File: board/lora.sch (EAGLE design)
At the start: 32 parts, among them IC1 STM32F030F4, IC2 ADP1607, J1 SWD_PTH_SHROUD, X1 SMA-142-0701-801/806, X2 UBLOX_MAX, X3 RFM98

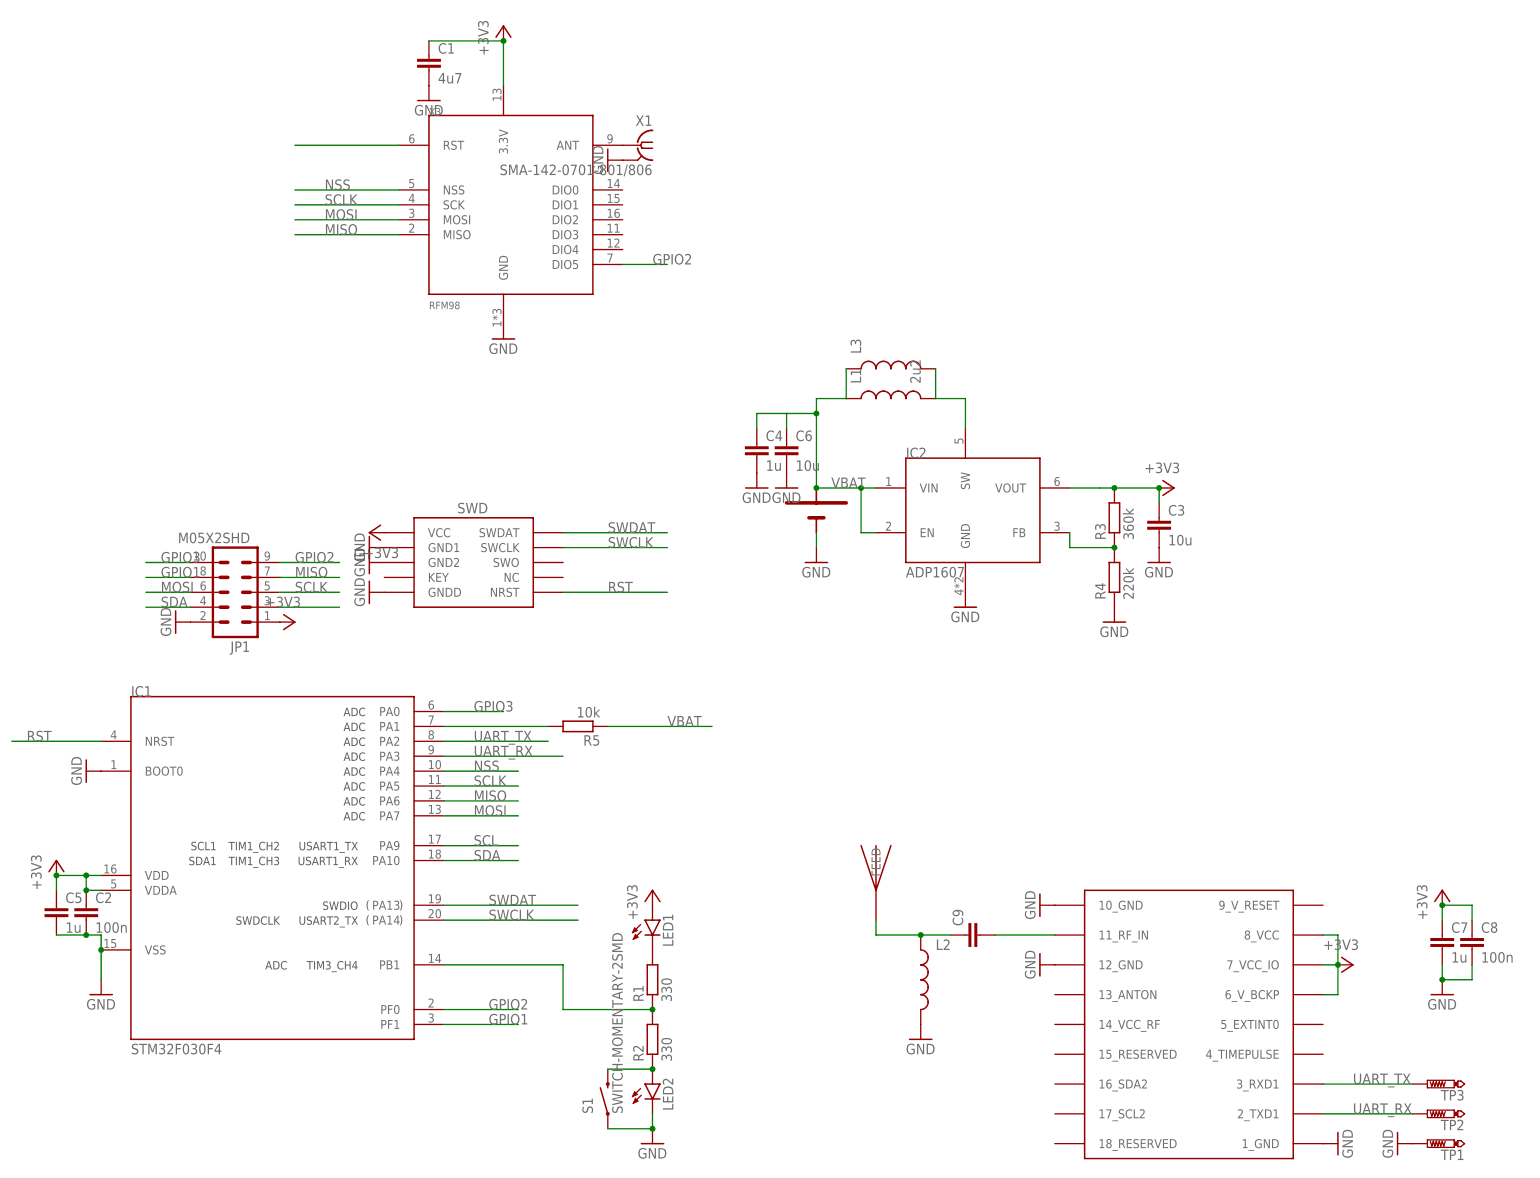
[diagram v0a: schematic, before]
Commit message: improvments
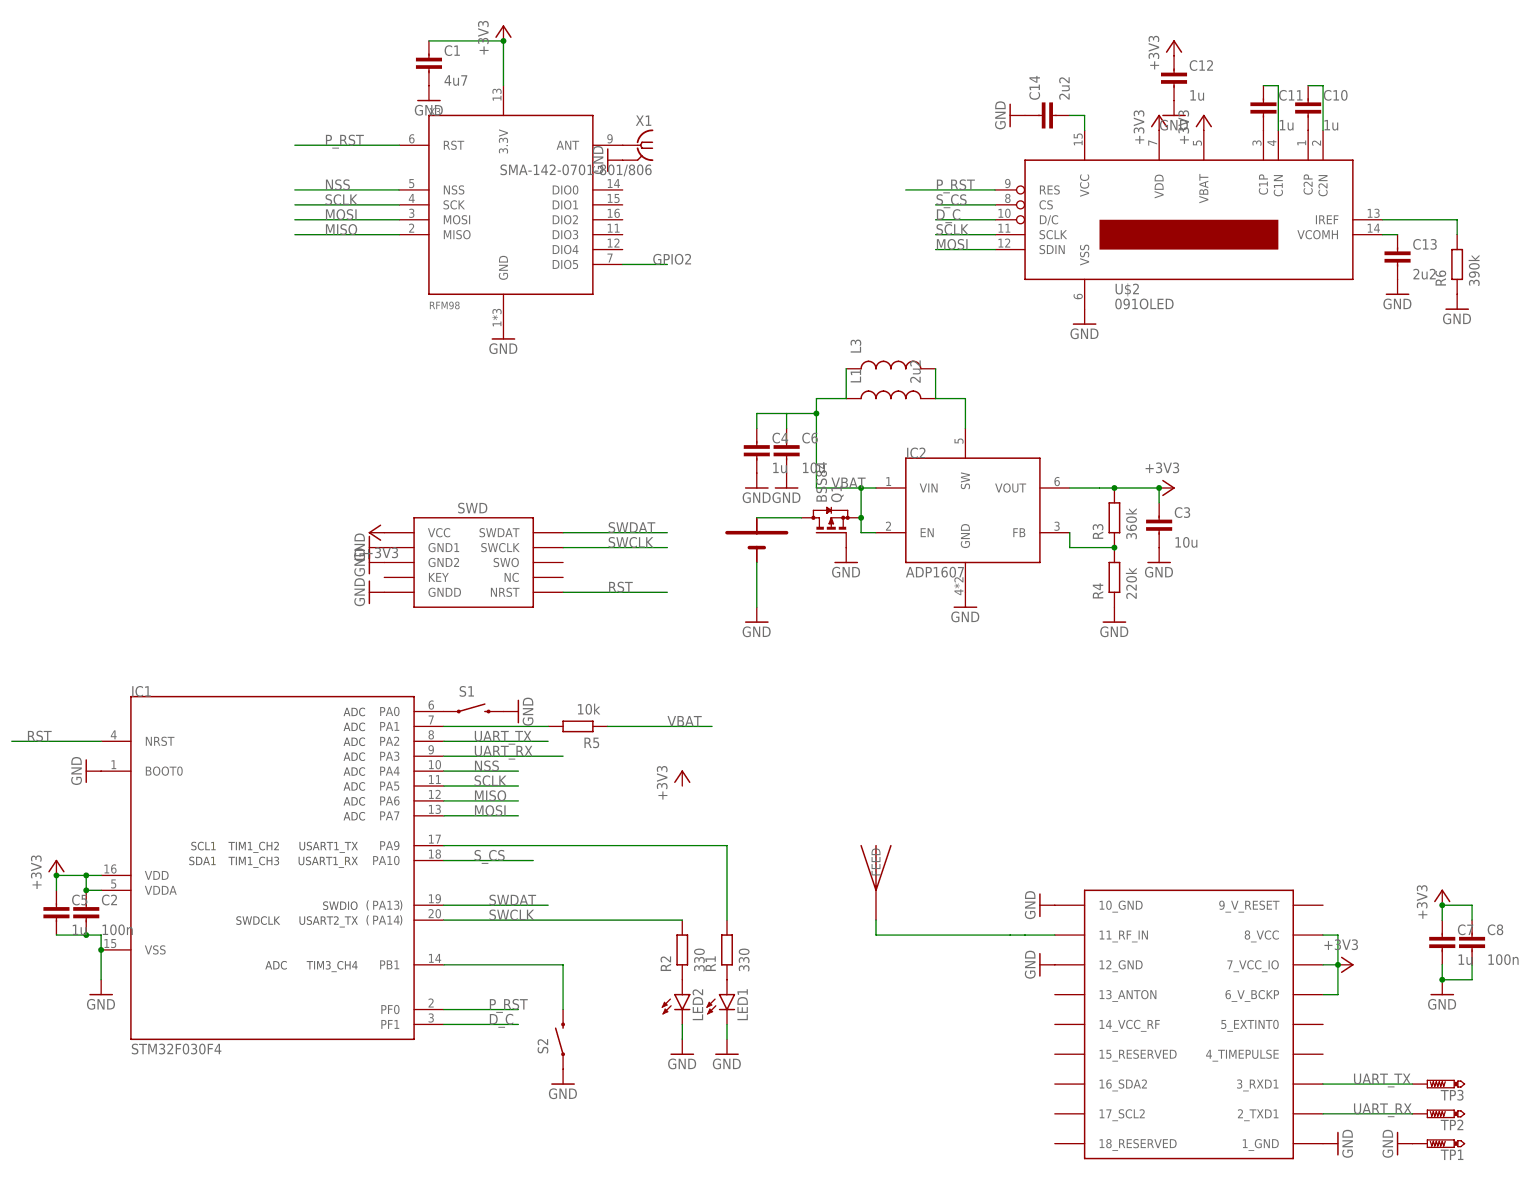
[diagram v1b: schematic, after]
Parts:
- removed C9: (no value), rcl:C-EUC0603
- removed JP1: M05X2SHD, SparkFun-Connectors:M05X2SHD
- removed L2: (no value), SparkFun-Passives:INDUCTOR0603
- added C10, C11, C12: 1u, passives-7351:CAPACITOR0603-N
- added C13, C14: 2u2, passives-7351:CAPACITOR0603-N
- added Q1: BSS84, transistor-small-signal:BSS84
- added R6: 390k, passives-7351:RESISTOR0603-N
- added S2: SWITCH-MOMENTARY-2SMD, Mine:SWITCH-MOMENTARY-2SMD
- added U$2: 091OLED, ukhas:091OLED
- C1, C2, C4, C5, C7, C8: device rcl:C-EUC0603 -> passives-7351:CAPACITOR0603-N
- C3, C6: device rcl:C-EUC0805 -> passives-7351:CAPACITOR0805-N
- R1, R2, R3, R4, R5: device rcl:R-EU_R0603 -> passives-7351:RESISTOR0603-N
- U$6: value KEYSTONE-53 -> KEYSTONE-92; device Mine:KEYSTONE-53 -> Mine:KEYSTONE-92
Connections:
- removed net GPIO1: IC1.PF1, JP1.8
- removed net GPIO3: IC1.PA0, JP1.10
- removed net N$10: X3.RST
- removed net SCL: IC1.PA9, JP1.3
- removed net SDA: IC1.PA10, JP1.4
- new net D_C: IC1.PF1, U$2.D/C
- new net N$11: C10.2, U$2.C2P
- new net N$12: C11.2, U$2.C1P
- new net N$13: C11.1, U$2.C1N
- new net N$14: C10.1, U$2.C2N
- new net N$15: C13.1, U$2.VCOMH
- new net N$16: R6.P$2, U$2.IREF
- new net N$18: IC1.PA0, S1.1
- new net N$20: IC1.PA9, R1.P$2
- new net P_RST: IC1.PF0, U$2.RES, X3.RST
- new net S_CS: IC1.PA10, U$2.CS
- new net VCC: C14.2, U$2.VCC
- net +3V3: now also C12.1, R3.P$2, U$2.VBAT, U$2.VDD; no longer JP1.1, LED1.A, R3.2
- net GND: now also C12.2, C13.2, C14.1, LED1.C, Q1.G, R4.P$1, R6.P$1, S1.2, S2.1, U$2.VSS; no longer JP1.2, L2.2, R4.1, S1.1
- net GPIO2: no longer IC1.PF0, JP1.9
- net MISO: no longer JP1.7
- net MOSI: now also U$2.SDIN; no longer JP1.6
- net N$1: now also LED1.A, R1.P$1; no longer C9.2, X2.11_RF_IN
- net N$4: now also X2.11_RF_IN; no longer C9.1, L2.1
- net N$5: now also R2.P$1; no longer R2.1, S1.2
- net N$6: now also R3.P$1, R4.P$2; no longer R3.1, R4.2
- net N$7: now also Q1.D, U$6.+; no longer LED1.C, R1.2
- net N$8: now also S2.2; no longer R1.1, R2.2
- net N$9: now also R5.P$2; no longer R5.2
- net SCLK: now also U$2.SCLK; no longer JP1.5
- net SWCLK: now also R2.P$2
- net VBAT: now also Q1.S, R5.P$1; no longer R5.1, U$6.+
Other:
- moved on the sheet: LED1, LED2, R1, R2, S1
